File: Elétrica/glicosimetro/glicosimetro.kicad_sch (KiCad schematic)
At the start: 19 parts, among them U1 ESP32-C3_SUPERMINI, U2 MCP6L01Rx-xOT, U3 MCP6L01Rx-xOT, U4 LM1117DT-3.3, U5 MCP6L01Rx-xOT, U6 MCP6L01Rx-xOT, U7 MCP6L01Rx-xOT

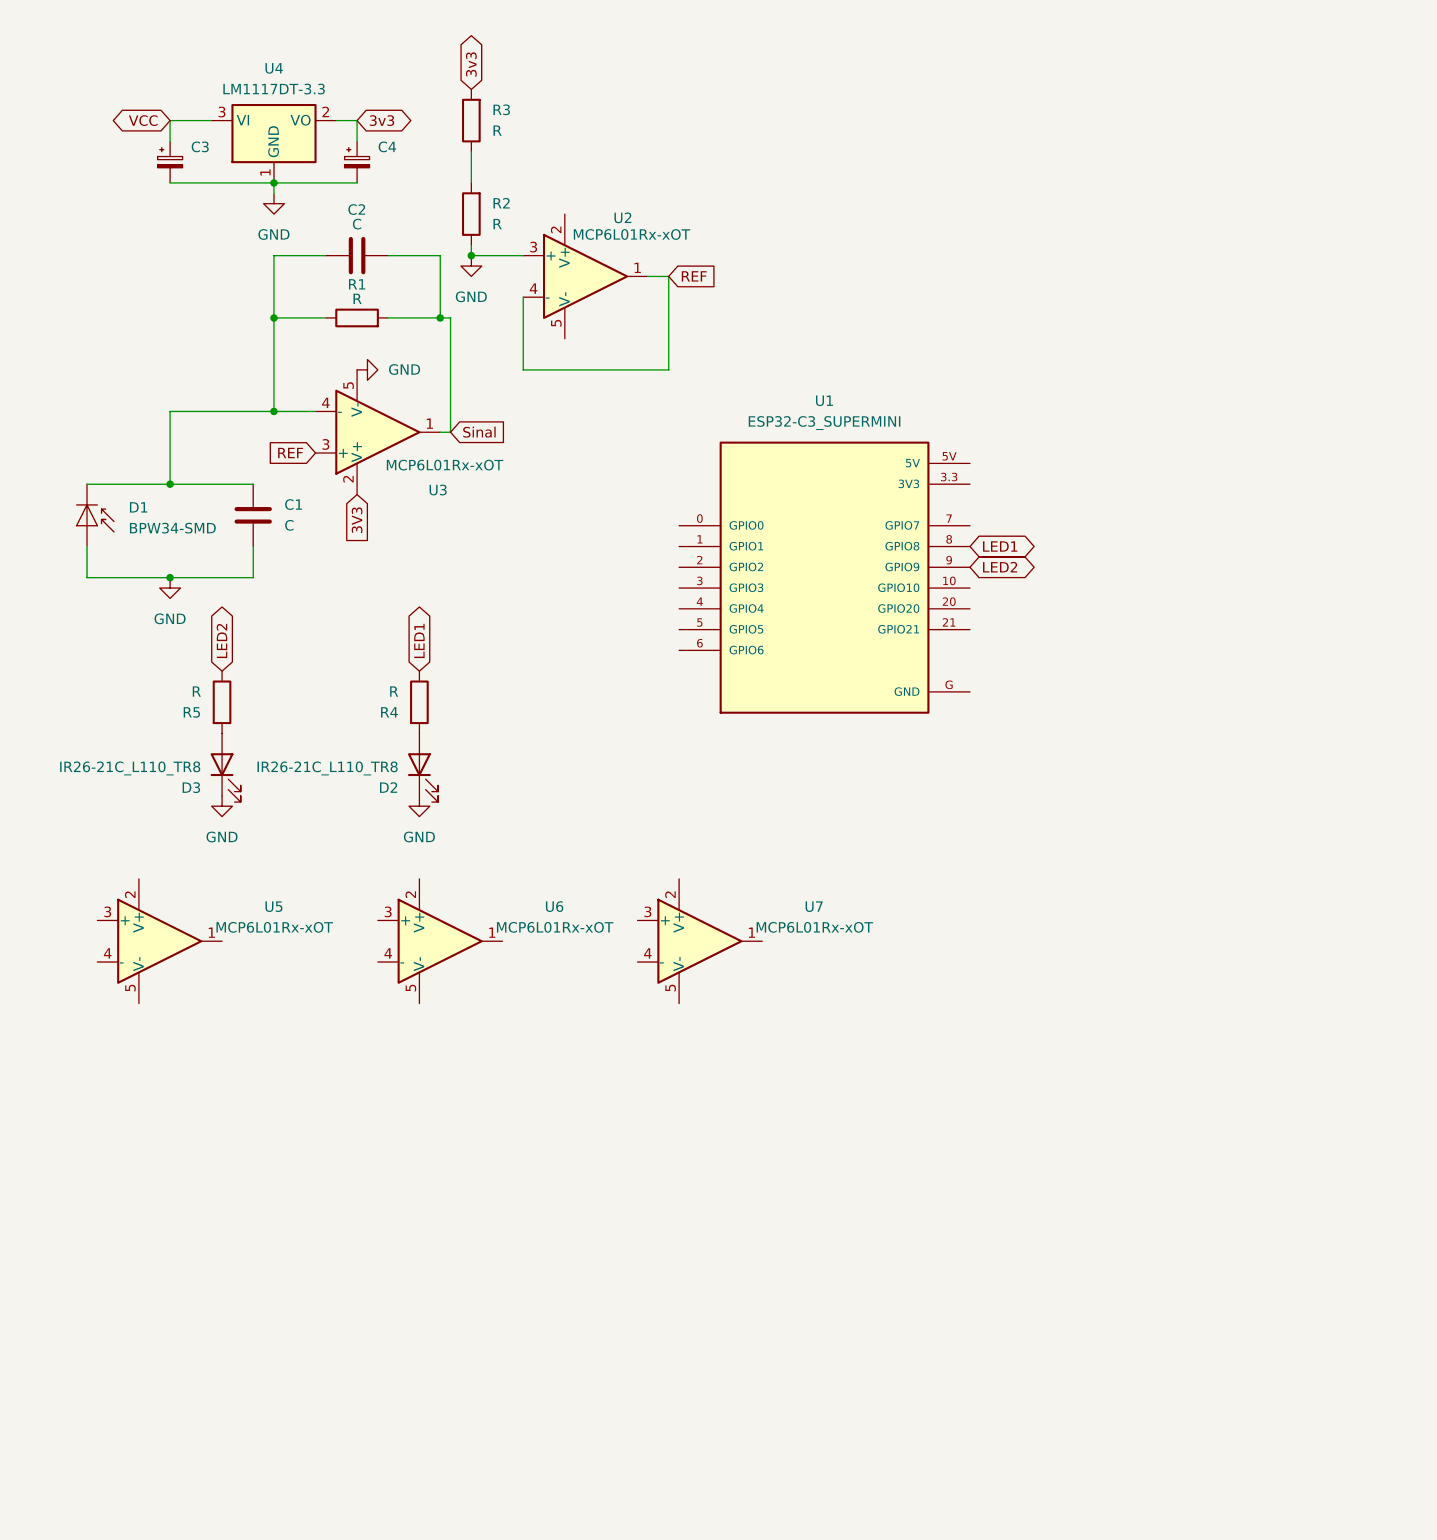
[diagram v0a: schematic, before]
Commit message: inicio da placa
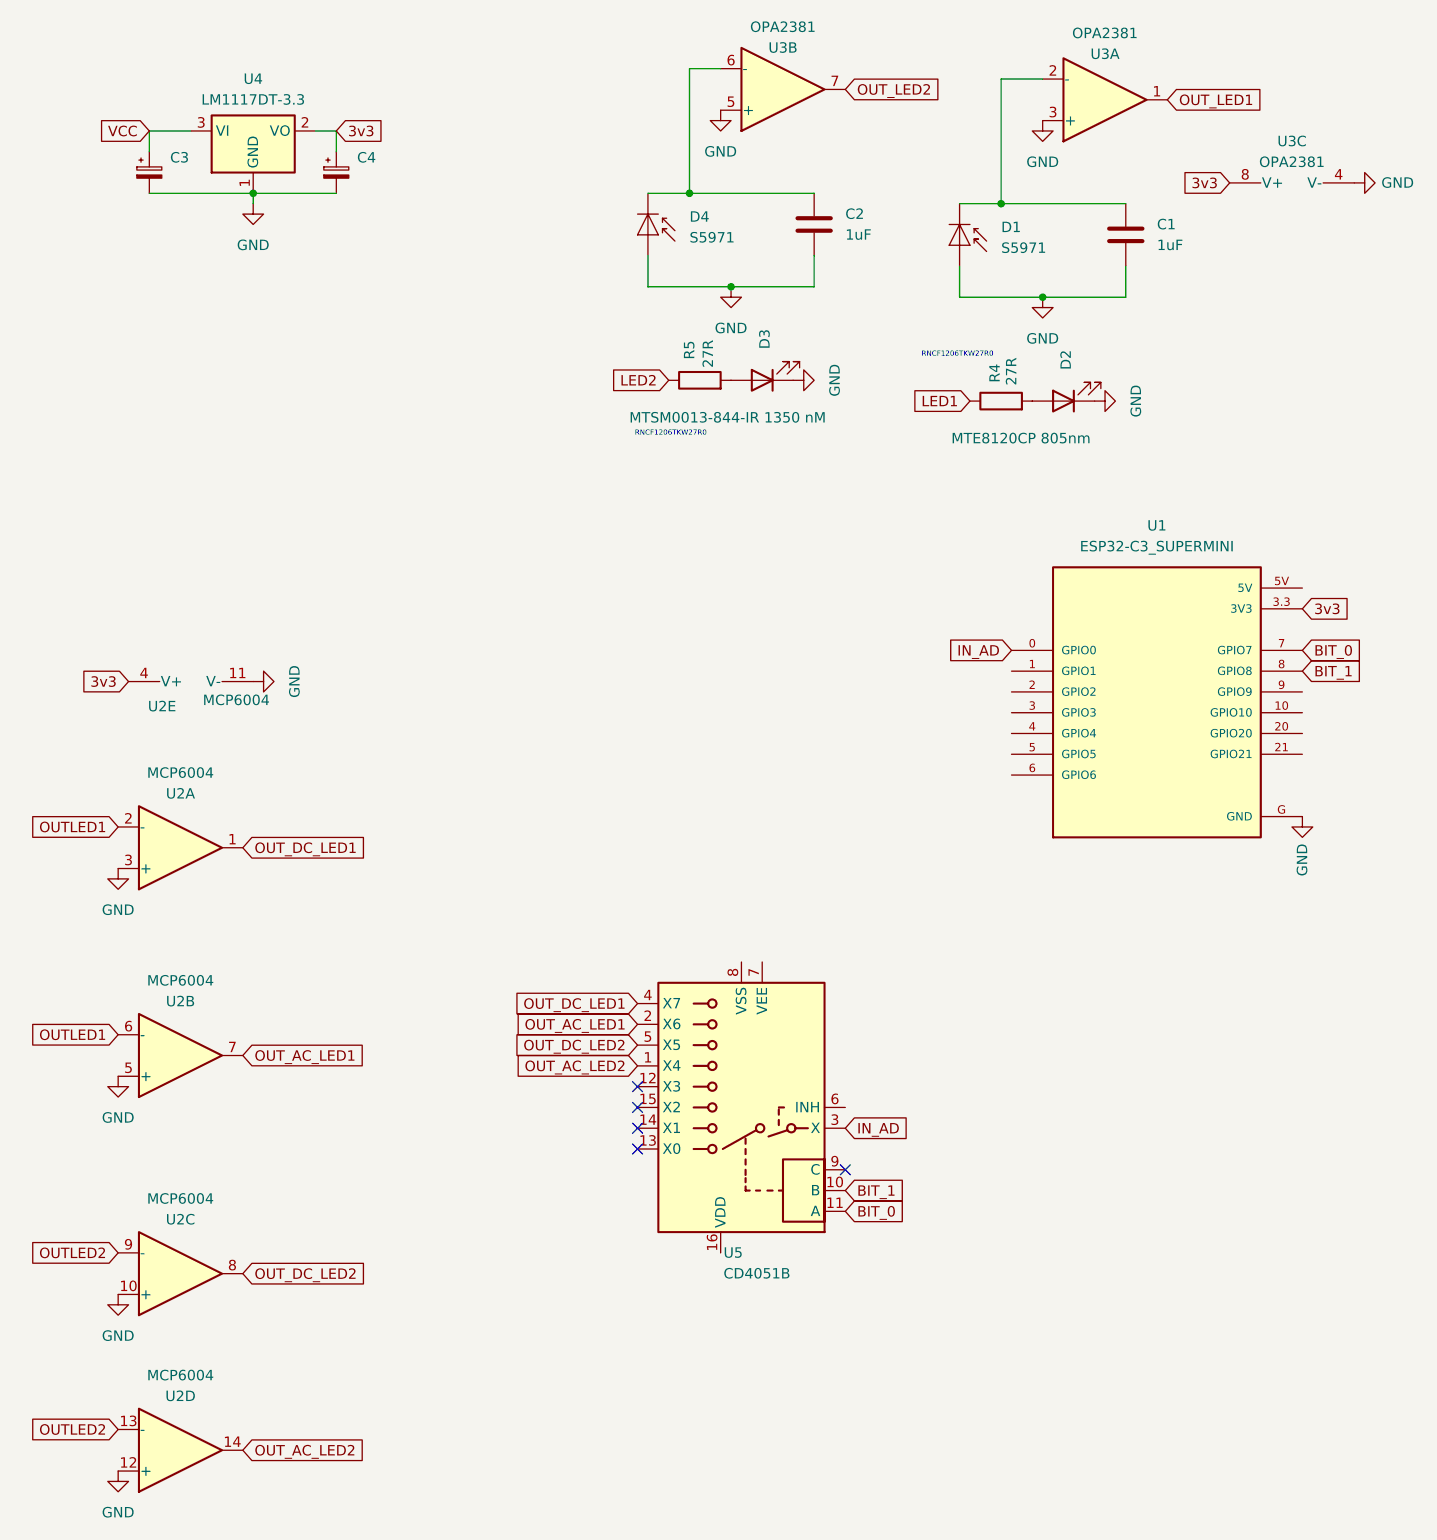
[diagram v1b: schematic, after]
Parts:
- removed R1, R2, R3: R, Resistor_SMD:R_0603_1608Metric_Pad0.98x0.95mm_HandSolder, symbol Device:R
- removed U2, U3, U5, U6, U7: MCP6L01Rx-xOT, Package_TO_SOT_SMD:SOT-23-5, symbol Amplifier_Operational:MCP6L01Rx-xOT
- added D4: S5971, OptoDevice:Osram_BPW34S-SMD, symbol Sensor_Optical:BPW34-SMD
- added U2: MCP6004, symbol Amplifier_Operational:MCP6004
- added U3: OPA2381, Package_SO:SOIC-8_3.9x4.9mm_P1.27mm, symbol Amplifier_Operational:OPA2340
- added U5: CD4051B, MUX:DIP794W45P254L1969H508Q16, symbol Analog_Switch:CD4051B
- C1, C2: value C -> 1uF
- D1: value BPW34-SMD -> S5971
- D2: value IR26-21C_L110_TR8 -> MTE8120CP 805nm
- D3: value IR26-21C_L110_TR8 -> MTSM0013-844-IR 1350 nM
- R4, R5: value R -> 27R
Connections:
- net Sinal is gone; now on net GND: C2.2
- net 3v3: now also U1.3.3 (3V3), U2.4 (V+), U3.8 (V+)
- net GND: now also U1.G (GND), D4.2 (A), U2.10 (+), U2.11 (V-), U2.12 (+), U2.3 (+), U2.5 (+), U3.3 (+), U3.4 (V-), U3.5 (+)
- net LED1: no longer U1.8 (GPIO8)
- net LED2: no longer U1.9 (GPIO9)
- net at C1.1, D1.1 (K): now also U3.2 (-); no longer C2.1
- net IN_AD: now reaches U1.0 (GPIO0)
- net IN_AD: now also U5.3 (X)
- net BIT_0: now reaches U1.7 (GPIO7)
- net BIT_0: now also U5.11 (A)
- new net: C2.1, D4.1 (K), U3.6 (-)
- new net BIT_1: U1.8 (GPIO8), U5.10 (B)
- new net OUTLED1: U2.2 (-), U2.6 (-)
- new net OUTLED2: U2.13 (-), U2.9 (-)
- new net OUT_AC_LED1: U2.7, U5.2 (X6)
- new net OUT_AC_LED2: U2.14, U5.1 (X4)
- new net OUT_DC_LED1: U2.1, U5.4 (X7)
- new net OUT_DC_LED2: U2.8, U5.5 (X5)
- new net OUT_LED1: U3.1
- new net OUT_LED2: U3.7
- no-connect marks 0 -> 5
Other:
- note added: "RNCF1206TKW27R0"
- moved on the sheet: C1, C3, C4, D1, D2, D3, R4, R5, U1, U4
